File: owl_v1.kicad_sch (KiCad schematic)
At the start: 17 parts, among them SW1 SW_SPDT, U1 STM32F103C8T6, Y1 8MHz, Y2 32k768

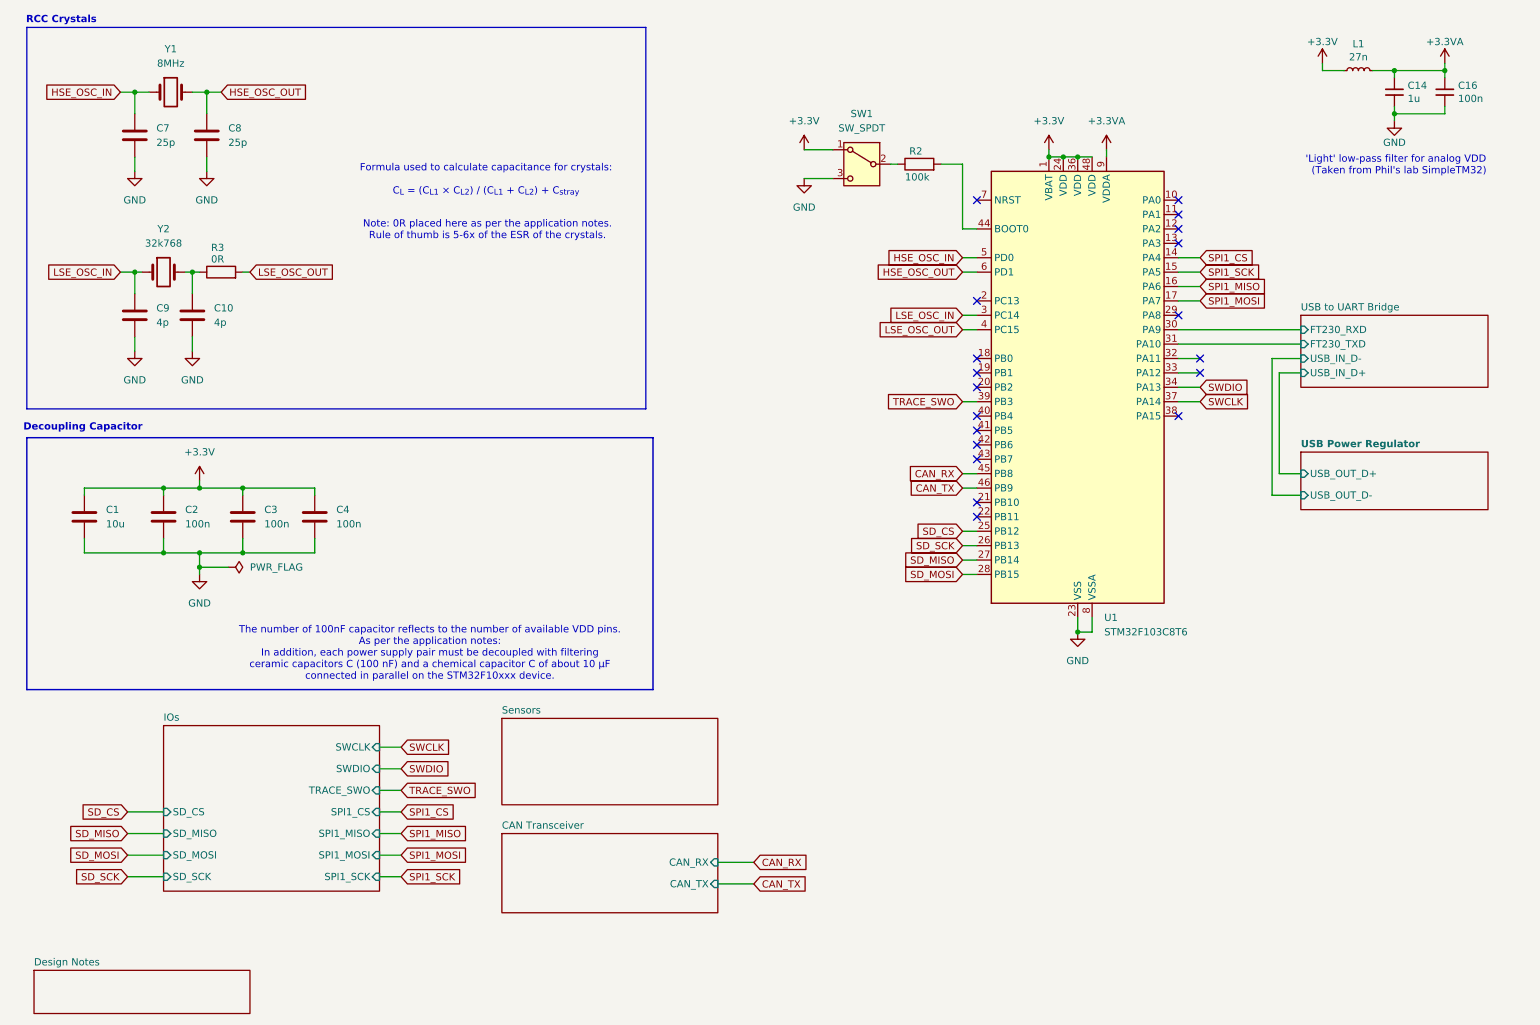
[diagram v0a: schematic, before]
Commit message: [feat] Add I2C breakout
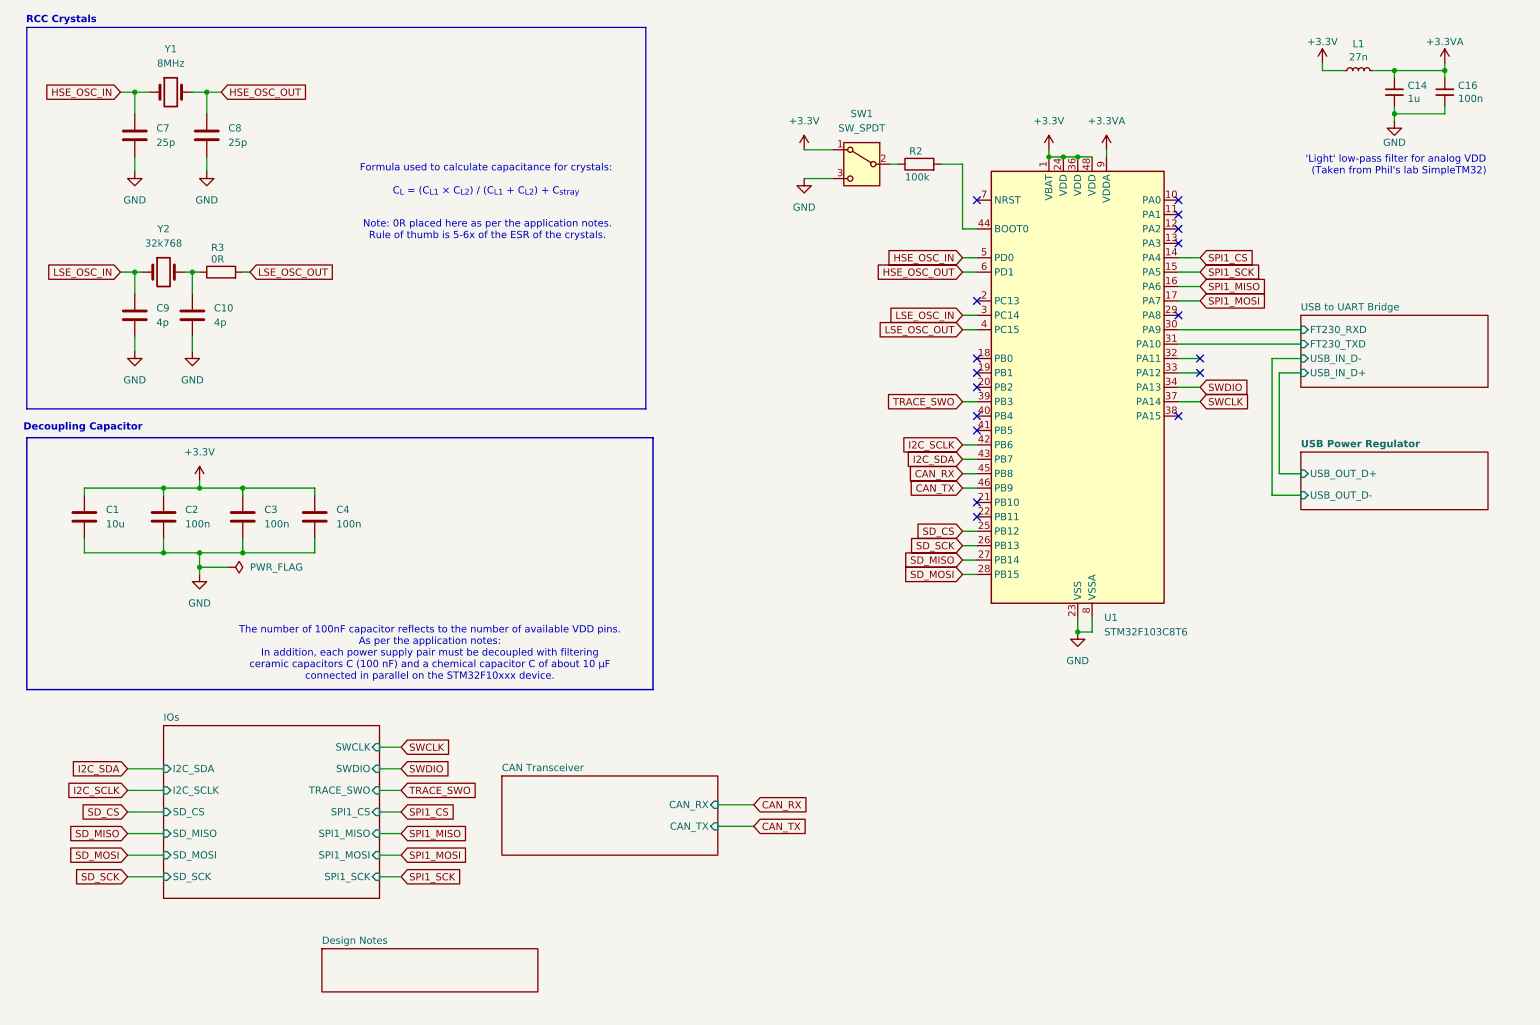
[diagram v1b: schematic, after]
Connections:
- net I2C_SCLK: now reaches U1.42 (PB6)
- net I2C_SDA: now reaches U1.43 (PB7)
- no-connect marks 19 -> 17
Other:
- removed sheet Sensors
- sheet IOs ports: added I2C_SCLK, I2C_SDA; removed none
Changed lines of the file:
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@@
 	)
 	(no_connect
-		(at 185.42 96.52)
-	)
-	(no_connect
 		(at 185.42 91.44)
 	)
@@
 	)
 	(no_connect
-		(at 185.42 93.98)
-	)
-	(no_connect
 		(at 185.42 106.68)
 	)
@@
 	(wire
 		(pts
-			(xy 139.7 171.45) (xy 146.05 171.45)
+			(xy 139.7 161.29) (xy 146.05 161.29)
 		)
 		(stroke
@@
 	(wire
 		(pts
+			(xy 182.88 96.52) (xy 185.42 96.52)
+		)
+		(stroke
+			(width 0)
+			(type default)
+		)
+	)
+	(wire
+		(pts
 			(xy 182.88 44.45) (xy 182.88 55.88)
 		)
@@
 	(wire
 		(pts
+			(xy 35.56 154.94) (xy 41.91 154.94)
+		)
+		(stroke
+			(width 0)
+			(type default)
+		)
+	)
+	(wire
+		(pts
 			(xy 27.94 101.6) (xy 27.94 102.87)
 		)
@@
 	(wire
 		(pts
-			(xy 139.7 167.64) (xy 146.05 167.64)
+			(xy 35.56 151.13) (xy 41.91 151.13)
+		)
+		(stroke
+			(width 0)
+			(type default)
+		)
+	)
+	(wire
+		(pts
+			(xy 139.7 157.48) (xy 146.05 157.48)
 		)
 		(stroke
@@
 	(wire
 		(pts
+			(xy 182.88 93.98) (xy 185.42 93.98)
+		)
+		(stroke
+			(width 0)
+			(type default)
+		)
+	)
+	(wire
+		(pts
 			(xy 259.08 36.83) (xy 259.08 35.56)
 		)
@@
 		)
 	)
+	(global_label "I2C_SDA"
+		(shape input)
+		(at 182.88 96.52 180)
+		(fields_autoplaced yes)
+		(effects
+			(font
+				(size 1.27 1.27)
+			)
+			(justify right)
+		)
+		(property "Intersheetrefs" "${INTERSHEET_REFS}"
+			(at 172.2748 96.52 0)
+			(hide yes)
+			(show_name no)
+			(do_not_autoplace no)
+			(effects
+				(font
+					(size 1.27 1.27)
+				)
+				(justify right)
+			)
+		)
+	)
 	(global_label "HSE_OSC_OUT"
 		(shape input)
@@
 		)
 	)
+	(global_label "I2C_SCLK"
+		(shape input)
+		(at 35.56 154.94 180)
+		(fields_autoplaced yes)
+		(effects
+			(font
+				(size 1.27 1.27)
+			)
+			(justify right)
+		)
+		(property "Intersheetrefs" "${INTERSHEET_REFS}"
+			(at 23.7453 154.94 0)
+			(hide yes)
+			(show_name no)
+			(do_not_autoplace no)
+			(effects
+				(font
+					(size 1.27 1.27)
+				)
+				(justify right)
+			)
+		)
+	)
 	(global_label "SD_SCK"
 		(shape input)
@@
 		)
 	)
+	(global_label "I2C_SDA"
+		(shape input)
+		(at 35.56 151.13 180)
+		(fields_autoplaced yes)
+		(effects
+			(font
+				(size 1.27 1.27)
+			)
+			(justify right)
+		)
+		(property "Intersheetrefs" "${INTERSHEET_REFS}"
+			(at 24.9548 151.13 0)
+			(hide yes)
+			(show_name no)
+			(do_not_autoplace no)
+			(effects
+				(font
+					(size 1.27 1.27)
+				)
+				(justify right)
+			)
+		)
+	)
 	(global_label "SD_SCK"
 		(shape input)
@@
 	(global_label "CAN_RX"
 		(shape input)
-		(at 146.05 167.64 0)
+		(at 146.05 157.48 0)
 		(fields_autoplaced yes)
 		(effects
@@
 		)
 		(property "Intersheetrefs" "${INTERSHEET_REFS}"
-			(at 156.1714 167.64 0)
+			(at 156.1714 157.48 0)
 			(hide yes)
 			(show_name no)
@@
 	(global_label "CAN_TX"
 		(shape input)
-		(at 146.05 171.45 0)
+		(at 146.05 161.29 0)
 		(fields_autoplaced yes)
 		(effects
@@
 		)
 		(property "Intersheetrefs" "${INTERSHEET_REFS}"
-			(at 155.869 171.45 0)
+			(at 155.869 161.29 0)
 			(hide yes)
 			(show_name no)
@@
 		)
 	)
+	(global_label "I2C_SCLK"
+		(shape input)
+		(at 182.88 93.98 180)
+		(fields_autoplaced yes)
+		(effects
+			(font
+				(size 1.27 1.27)
+			)
+			(justify right)
+		)
+		(property "Intersheetrefs" "${INTERSHEET_REFS}"
+			(at 171.0653 93.98 0)
+			(hide yes)
+			(show_name no)
+			(do_not_autoplace no)
+			(effects
+				(font
+					(size 1.27 1.27)
+				)
+				(justify right)
+			)
+		)
+	)
 	(symbol
 		(lib_id "Device:C")
@@
 	)
 	(sheet
-		(at 101.6 162.56)
+		(at 101.6 152.4)
 		(size 38.1 13.97)
 		(exclude_from_sim no)
@@
 		)
 		(property "Sheetname" "CAN Transceiver"
-			(at 101.6 161.8484 0)
+			(at 101.6 151.6884 0)
 			(show_name no)
 			(do_not_autoplace no)
@@
 		)
 		(property "Sheetfile" "can_controller.kicad_sch"
-			(at 101.6 177.1146 0)
+			(at 101.6 166.9546 0)
 			(hide yes)
 			(show_name no)
@@
 		)
 		(pin "CAN_RX" input
-			(at 139.7 167.64 0)
+			(at 139.7 157.48 0)
 			(effects
 				(font
@@
 		)
 		(pin "CAN_TX" input
-			(at 139.7 171.45 0)
+			(at 139.7 161.29 0)
 			(effects
 				(font
@@
 	)
 	(sheet
-		(at 19.05 186.69)
+		(at 69.85 182.88)
 		(size 38.1 7.62)
 		(exclude_from_sim no)
@@
 		)
 		(property "Sheetname" "Design Notes"
-			(at 19.05 185.9784 0)
+			(at 69.85 182.1684 0)
 			(show_name no)
 			(do_not_autoplace no)
@@
 		)
 		(property "Sheetfile" "design_notes.kicad_sch"
-			(at 19.05 194.8946 0)
+			(at 69.85 191.0846 0)
 			(hide yes)
 			(show_name no)
@@
 	(sheet
 		(at 41.91 143.51)
-		(size 38.1 29.21)
+		(size 38.1 30.48)
 		(exclude_from_sim no)
 		(in_bom yes)
@@
 		)
 		(property "Sheetfile" "GPIOs.kicad_sch"
-			(at 41.91 173.3046 0)
+			(at 41.91 174.5746 0)
 			(hide yes)
 			(show_name no)
@@
 			)
 		)
+		(pin "I2C_SCLK" input
+			(at 41.91 154.94 180)
+			(effects
+				(font
+					(size 1.27 1.27)
+				)
+				(justify left)
+			)
+		)
+		(pin "I2C_SDA" input
+			(at 41.91 151.13 180)
+			(effects
+				(font
+					(size 1.27 1.27)
+				)
+				(justify left)
+			)
+		)
 		(instances
 			(project "owl_v1"
@@
 				)
 			)
-		)
-	)
-	(sheet
-		(at 101.6 142.24)
-		(size 38.1 15.24)
-		(exclude_from_sim no)
-		(in_bom yes)
-		(on_board yes)
-		(dnp no)
-		(fields_autoplaced yes)
-		(stroke
-			(width 0.1524)
-			(type solid)
-		)
-		(fill
-			(color 0 0 0 0)
-		)
-		(property "Sheetname" "Sensors"
-			(at 101.6 141.5284 0)
-			(show_name no)
-			(do_not_autoplace no)
-			(effects
-				(font
-					(size 1.27 1.27)
-				)
-				(justify left bottom)
-			)
-		)
-		(property "Sheetfile" "sensors.kicad_sch"
-			(at 101.6 158.0646 0)
-			(hide yes)
-			(show_name no)
-			(do_not_autoplace no)
-			(effects
-				(font
-					(size 1.27 1.27)
-				)
-				(justify left top)
-			)
-		)
-		(instances
-			(project "owl_v1"
-				(path "/c1d8d3e2-84ea-437a-bbb1-a2e651deb7ac"
-					(page "5")
-				)
-			)
